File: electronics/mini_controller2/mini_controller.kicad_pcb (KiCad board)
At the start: 4 copper layers, 13.2 x 60.6 mm, 50 parts, among them J1 terminal 1, J2 terminal 2, J3 sma, J4 Conn_01x04, J5 SWD port, Q1 MMBT3904, SW1 chs-01a, U1 JST-RCY, U10 SKY65723-81, U12 ADXL343, U2 BD33GA5WEFJ, U3 NCV51460, U4 MAX-M8C, U5 Si7232DN, U6 Si7232DN, U7 W25Q16JVS, U8 s76s, U9 MS5607-02BA, j1 power

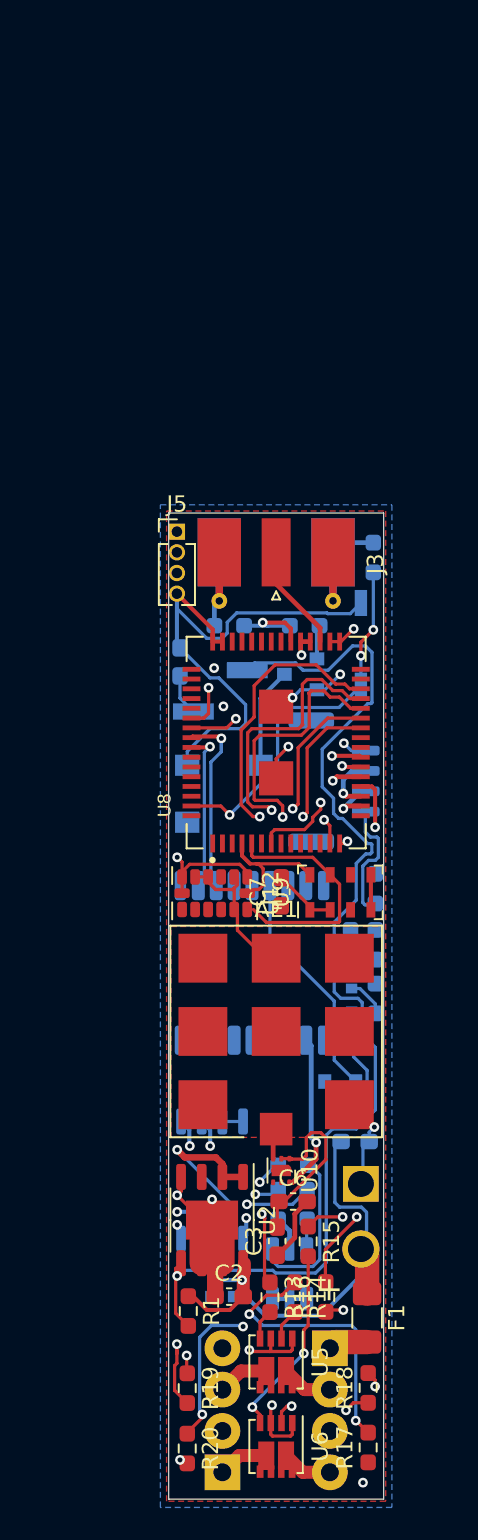
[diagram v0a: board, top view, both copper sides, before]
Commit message: mini controller finished
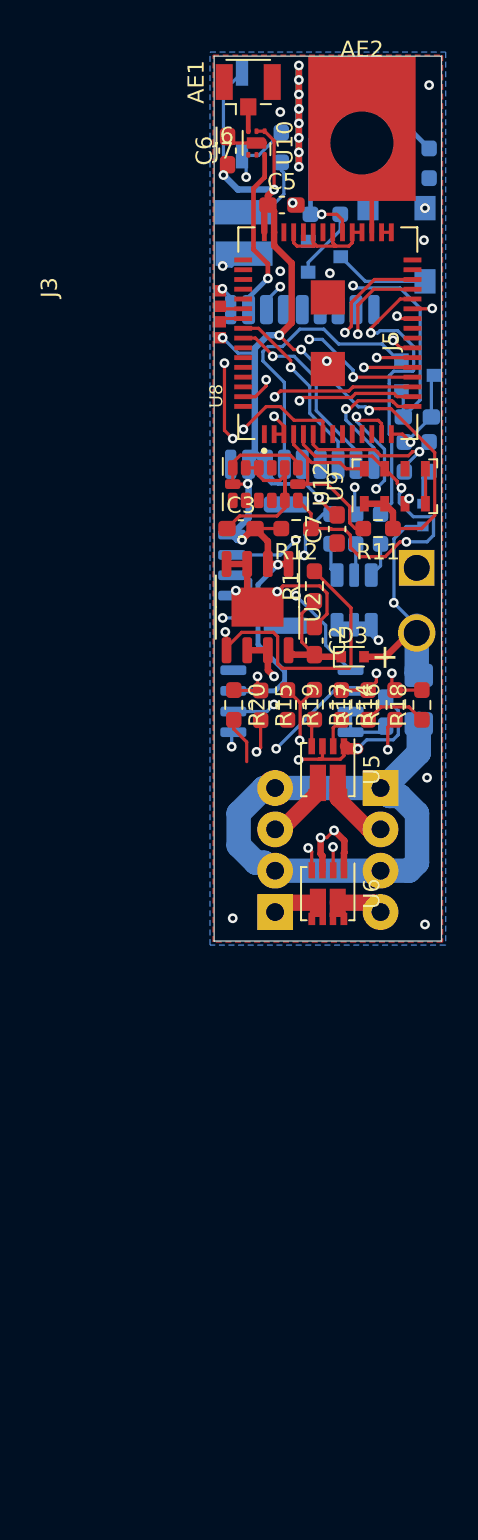
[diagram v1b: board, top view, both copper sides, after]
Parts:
- added AE2: ANT-868-PW-LP, custom:ANT-868-PW-LP, F.Cu at (136.1, 39.9)
- added C4: 0.1u, Capacitor_SMD:C_0603_1608Metric_Pad1.08x0.95mm_HandSolder, B.Cu at (137.5, 74.8)
- added J6: SWDIO, custom:just_a_pad, F.Cu at (127.5, 49.7)
- added J7: SWCLK, custom:just_a_pad, F.Cu at (127.5, 50.7)
- AE1: value SGGP.12A -> U.FL; footprint custom:SGGP.12.4.A.02 -> Connector_Coaxial:U.FL_Hirose_U.FL-R-SMT-1_Vertical
- C5, D3, R11, R12: moved to F.Cu
- F1: moved to B.Cu
- J3: value sma -> GND; footprint Connector_Coaxial:SMA_Molex_73251-2120_EdgeMount_Horizontal -> custom:just_a_pad
- J5: value SWD port -> 3V3; footprint Connector_PinHeader_1.27mm:PinHeader_1x04_P1.27mm_Vertical -> custom:just_a_pad
- j1: footprint Connector_PinHeader_2.54mm:PinHeader_1x02_P2.54mm_Vertical_SMD_Pin1Left -> custom:PinHeader_1x02_P2.54mm_Vertical_SMD
- moved C6 64.7 mm to (127.8, 40.3), turned to 90 degrees
- moved AE1 63.9 mm to (129.1, 36.6), turned to 90 degrees
- moved U10 63.1 mm to (129.6, 39.9)
- moved R20 45.8 mm to (128.2, 74.4)
- moved R17 45.6 mm to (136.5, 74.4)
- moved R1 45.2 mm to (133.2, 67.1), turned to 90 degrees
- moved C1 44.7 mm to (139.5, 56.7)
- moved U3 44.6 mm to (139.5, 54.1), turned to 0 degrees
- moved C3 43.8 mm to (128.7, 63.6), turned to 0 degrees
- moved R19 42.4 mm to (131.5, 74.4)
- moved R18 42.1 mm to (139.8, 74.4)
- moved R3 41.8 mm to (135.7, 63.6), turned to 270 degrees
- moved R4 41.7 mm to (137.2, 63.6)
- moved D2 41.6 mm to (135.6, 67.9)
- moved C2 40.6 mm to (133.2, 70.4), turned to 270 degrees
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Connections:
- J3 pad 1: Net-(J3-Pad1) -> GND
- J5 pad 1: GND -> /3V3
- R3 pad 1: Net-(D2-Pad2) -> /LED_R
- R3 pad 2: /LED_R -> Net-(D2-Pad2)
- U8 pad 26: /LED_B -> /LED_G
- U8 pad 28: /LED_G -> /LED_B
- U8 pad 33: Net-(J3-Pad1) -> Net-(AE2-Pad1)
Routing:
- net GND: track 64.3 -> 115.7 mm, vias 19 -> 32
- net /PYRO_3_EN: track 55.8 -> 24.7 mm, vias 4 -> 2
- net /PYRO_2_EN: track 58.6 -> 28.3 mm, vias 3 -> 2
- net /LED_G: track 46.4 -> 18.6 mm, vias 2 -> 1
- net /EXT_RX: track 3.60 -> 28.9 mm, vias 1 -> 2
- net Net-(R1-Pad2): track 68.9 -> 44.1 mm, vias 1 -> 4
- net /PYRO_4_EN: track 45.7 -> 22.6 mm
- net Net-(C1-Pad2): track 30.6 -> 52.9 mm, vias 0 -> 2
- net /LED_R: track 43.3 -> 21.4 mm
- net /EXT_TX: track 2.96 -> 20.2 mm, vias 1 -> 2
- net /LED_B: track 42.1 -> 25.5 mm
- net /PYRO_1_EN: track 53.9 -> 40.2 mm, vias 3 -> 2
- net /SWCLK: track 15.1 -> 1.49 mm, vias 1 -> 0
- net /FLASH_MISO: track 41.4 -> 30.5 mm
- net /BUZZER: track 5.88 -> 16.7 mm
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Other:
- board size 13.2 x 60.6 mm -> 14 x 54.4 mm
